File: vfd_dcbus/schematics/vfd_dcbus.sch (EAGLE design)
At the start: 49 parts, among them J10 VT FS-P 6,35, J11 VT FS-P 6,35, J12 VT FS-P 6,35, J13 VT FS-PW 6,35, J14 VT FS-P 6,35, J15 VT FS-P 6,35, J16 VT FS-PW 6,35, J17 VT FS-P 6,35, J18 VT FS-P 6,35, J19 VT FS-P 6,35, J20 VT FS-P 6,35, J21 VT FS-P 6,35, J22 VT FS-P 6,35, J23 VT FS-P 6,35, J24 VT FS-P 6,35, J25 VT FS-PW 6,35, J26 VT FS-P 6,35, J27 VT FS-P 6,35, J28 VT FS-P 6,35, J29 VT FS-P 6,35, J3 VT FS-PW 6,35, J30 VT FS-P 6,35, J31 VT FS-P 6,35, J4 VT FS-P 6,35, J5 VT FS-P 6,35, J6 VT FS-PW 6,35, J7 VT FS-P 6,35, J8 VT FS-P 6,35, J9 VT FS-P 6,35, X1 JST XH2P ST, X2 JST XH2P ST, X3 JST XH2P ST, X4 JST XH2P ST, X5 JST XH2P ST

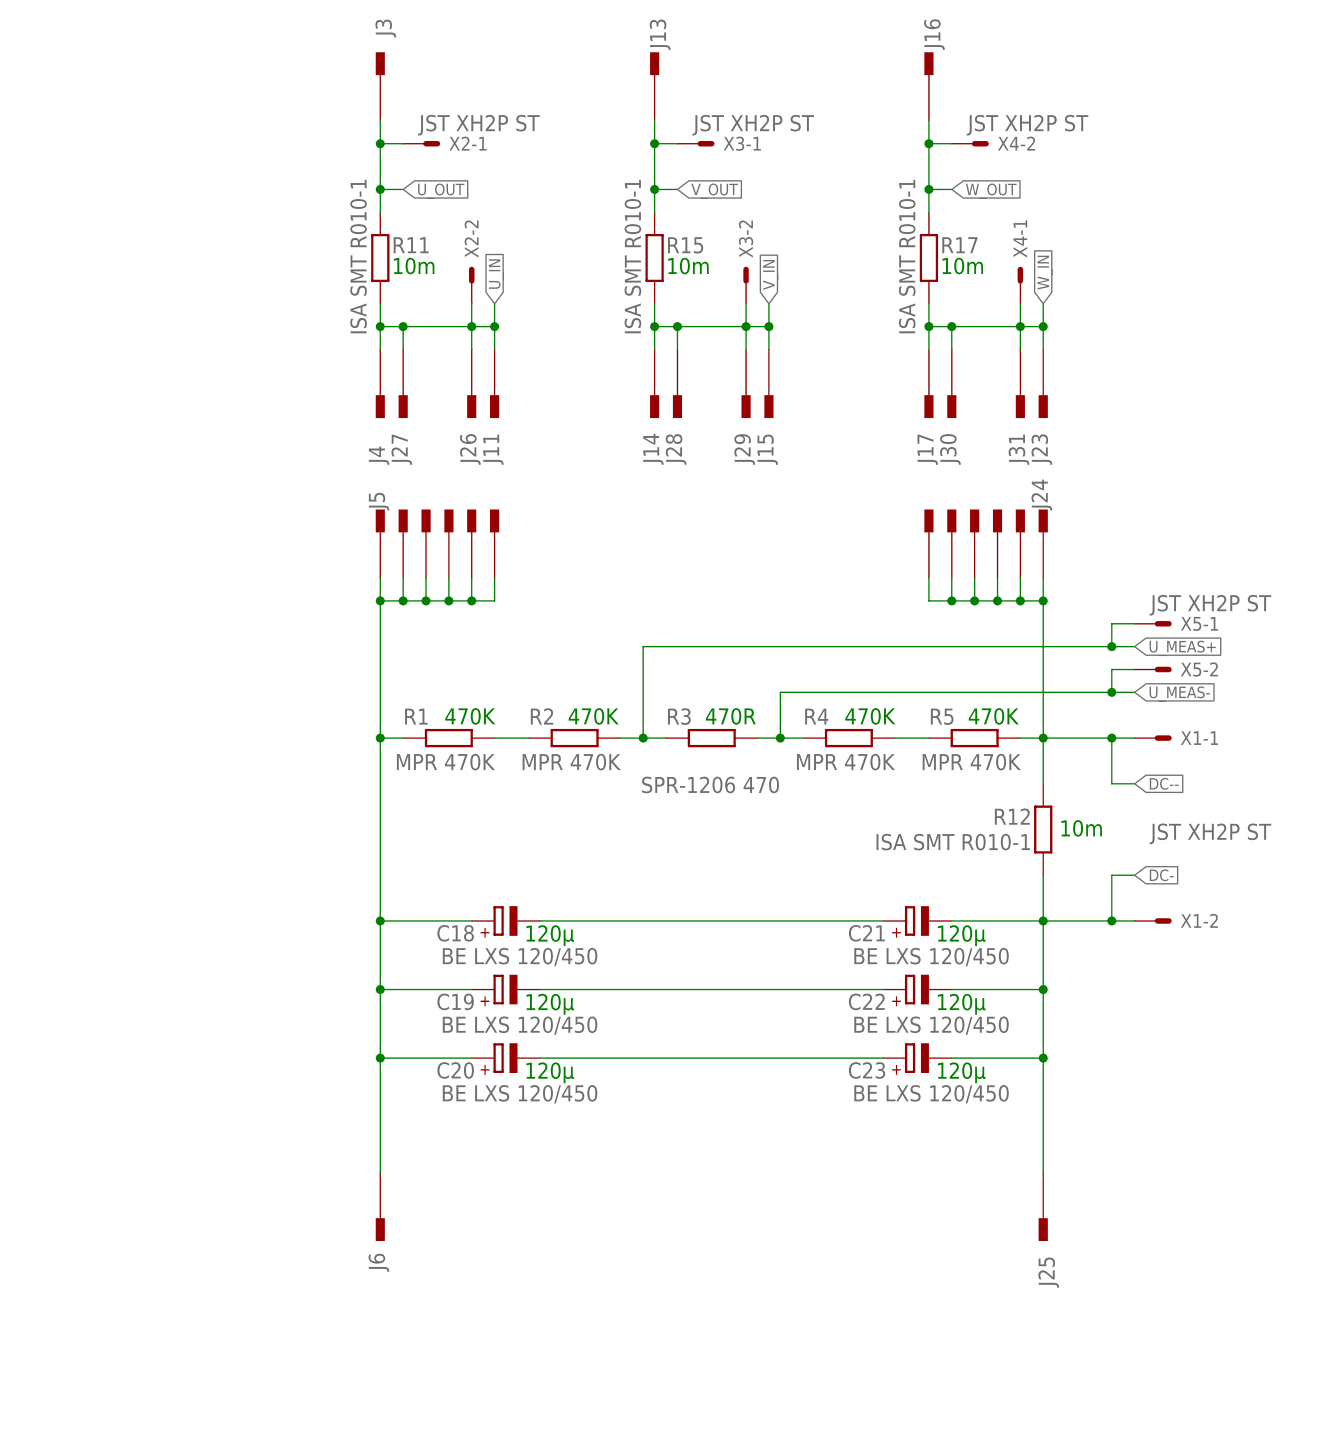
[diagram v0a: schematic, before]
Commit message: Updated Schematics
Updated already finnished schematics with Reichelt (DE) parts attribute

Finalized the controller board
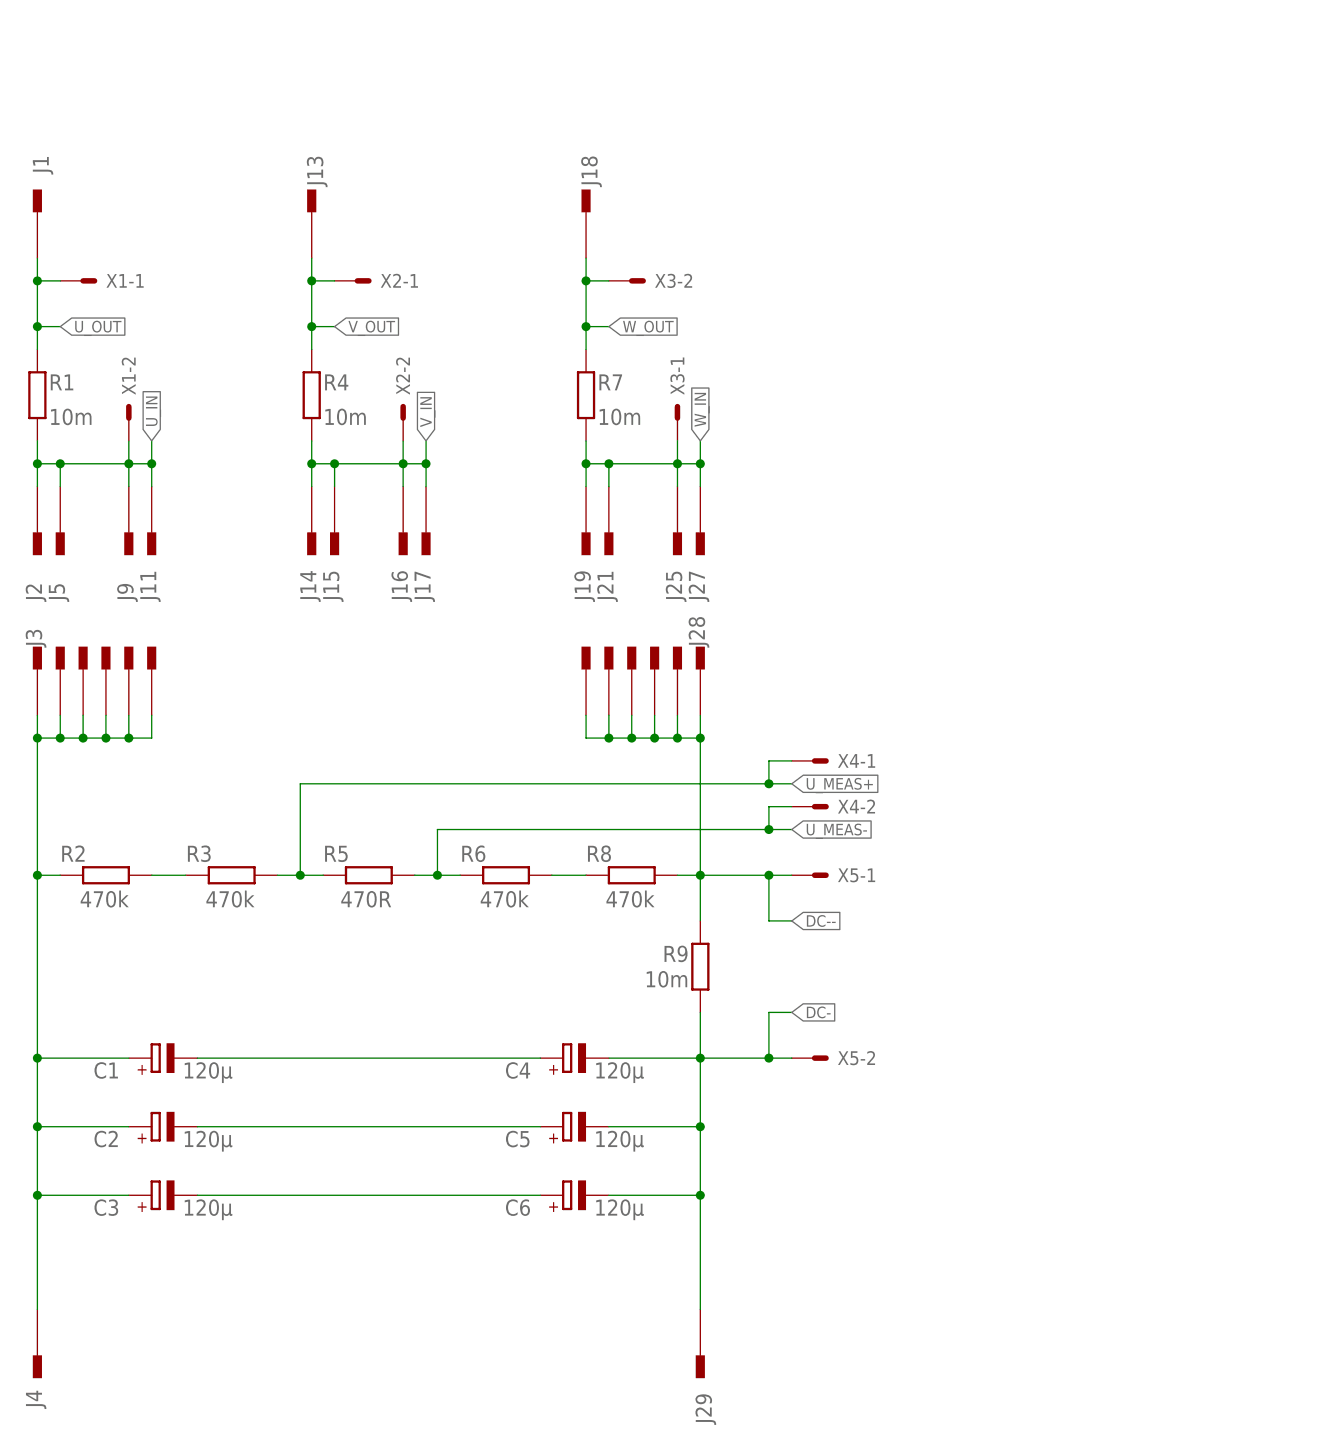
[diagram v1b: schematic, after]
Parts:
- removed C18, C19, C20, C21, C22, C23: BE LXS 120/450, resistor:CPOL-EUE10-25
- removed J30, J31: VT FS-P 6,35, con-faston:PIN2F061.080
- removed R11, R12, R15, R17: ISA SMT R010-1, resistor:R-EU_R2512
- added C1, C2, C3, C4, C5, C6: 120µ, resistor:CPOL-EUE10-25
- added J1: PIN2F061.200, con-faston:PIN2F061.200
- added J2: PIN2F061.080, con-faston:PIN2F061.080
- added R6, R8: 470k, rcl:R-EU_0207/5V
- added R7, R9: 10m, resistor:R-EU_R2512
- J10, J11, J12, J14, J15, J17, J19, J20, J21, J22, J23, J24, J26, J27, J28, J5, J7, J8, J9: value VT FS-P 6,35 -> PIN2F061.080; R (none) -> VT FS-P 6,35
- J13: value VT FS-PW 6,35 -> PIN2F061.200; R (none) -> VT FS-PW 6,35
- J16, J25, J3, J6: value VT FS-PW 6,35 -> PIN2F061.080; device con-faston:PIN2F061.200 -> con-faston:PIN2F061.080; R (none) -> VT FS-P 6,35
- J18, J29, J4: value VT FS-P 6,35 -> PIN2F061.200; device con-faston:PIN2F061.080 -> con-faston:PIN2F061.200; R (none) -> VT FS-PW 6,35
- R1, R4: value MPR 470K -> 10m; device rcl:R-EU_0207/5V -> resistor:R-EU_R2512; R (none) -> ISA SMT R010-1
- R2: value MPR 470K -> 470k; R (none) -> MPR 470K
- R3: value SPR-1206 470 -> 470k; device rcl:R-EU_R1206 -> rcl:R-EU_0207/5V; R (none) -> MPR 470K
- R5: value MPR 470K -> 470R; device rcl:R-EU_0207/5V -> rcl:R-EU_R1206; R (none) -> SPR-1206 470
- X1, X2, X3, X4, X5: value JST XH2P ST -> JST-XH-02-PIN-LONG-PAD; R (none) -> JST XH2P ST
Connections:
- net DC+: now also C1.+, C2.+, C3.+, J3.1, J4.1, R2.2; no longer C18.+, C19.+, C20.+, J5.1, J9.1, R1.2
- net DC-: now also C4.-, C5.-, C6.-, J29.1, R9.1, X5-2.S; no longer C21.-, C22.-, C23.-, J25.1, R12.1, X1-2.S
- net DC--: now also J23.1, J26.1, J28.1, R8.2, R9.2, X5-1.S; no longer J18.1, J19.1, J21.1, R12.2, R5.2, X1-1.S
- net N$1: now also R3.1; no longer R1.1
- net N$10: now also C3.-, C6.+; no longer C20.-, C23.+
- net N$2: now also R6.1, R8.1; no longer R4.1, R5.1
- net N$8: now also C1.-, C4.+; no longer C18.-, C21.+
- net N$9: now also C2.-, C5.+; no longer C19.-, C22.+
- net U_IN: now also J2.1, J5.1, J9.1, R1.1, X1-2.S; no longer J26.1, J27.1, J4.1, R11.1, X2-2.S
- net U_MEAS+: now also R3.2, R5.1, X4-1.S; no longer R2.2, R3.1, X5-1.S
- net U_MEAS-: now also R5.2, R6.2, X4-2.S; no longer R3.2, R4.2, X5-2.S
- net U_OUT: now also J1.1, R1.2, X1-1.S; no longer J3.1, R11.2, X2-1.S
- net V_IN: now also J16.1, J17.1, R4.1, X2-2.S; no longer J28.1, J29.1, R15.1, X3-2.S
- net V_OUT: now also R4.2, X2-1.S; no longer R15.2, X3-1.S
- net W_IN: now also J19.1, J21.1, J25.1, J27.1, R7.1, X3-1.S; no longer J17.1, J23.1, J30.1, J31.1, R17.1, X4-1.S
- net W_OUT: now also J18.1, R7.2, X3-2.S; no longer J16.1, R17.2, X4-2.S
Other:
- note removed: "10m"
- note removed: "120µ"
- note removed: "470K"
- note removed: "470R"
- moved on the sheet: J11, J13, J14, J15, J16, J17, J25, J27, J28, J29, J3, J4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
